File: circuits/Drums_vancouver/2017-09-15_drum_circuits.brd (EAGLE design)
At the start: 32 x 46 mm, 32 parts, among them IC2 MIC5225-5v, U2 ATMEGA328P_TQFP

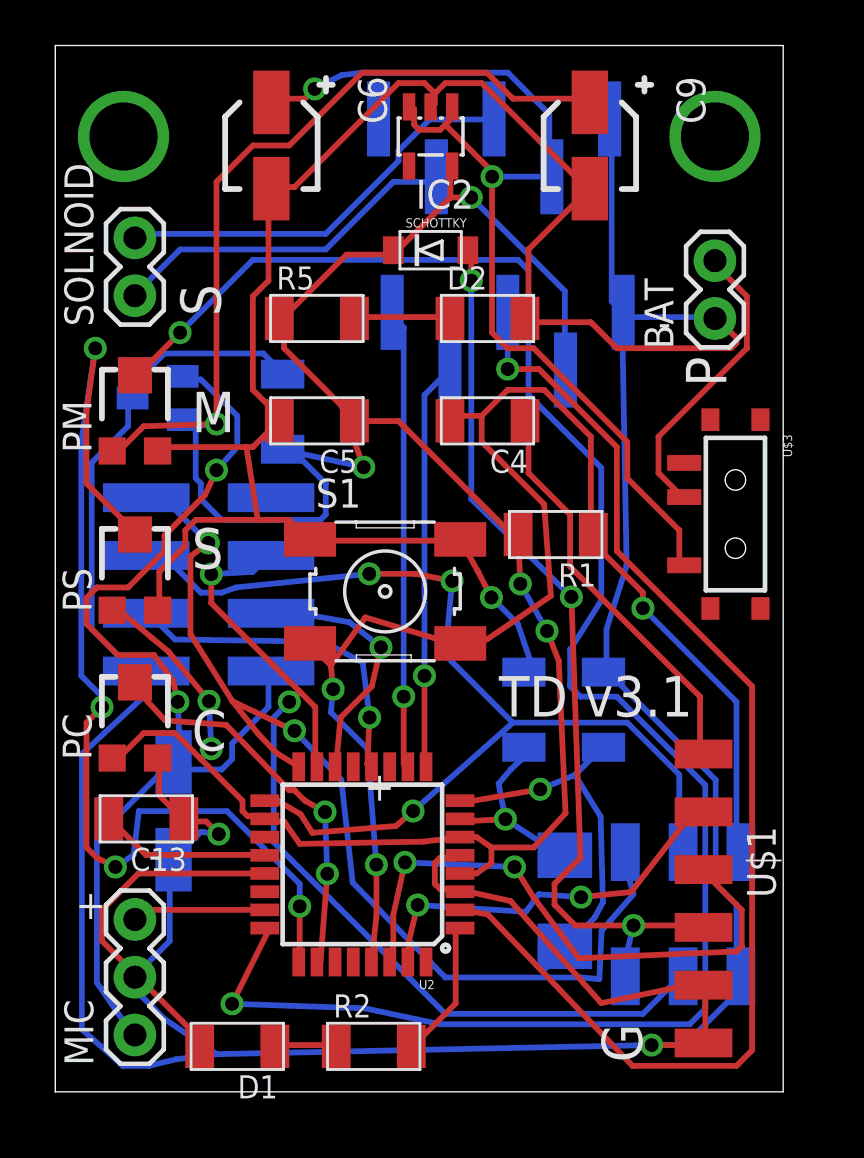
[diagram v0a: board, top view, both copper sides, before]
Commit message: updated slave, communication
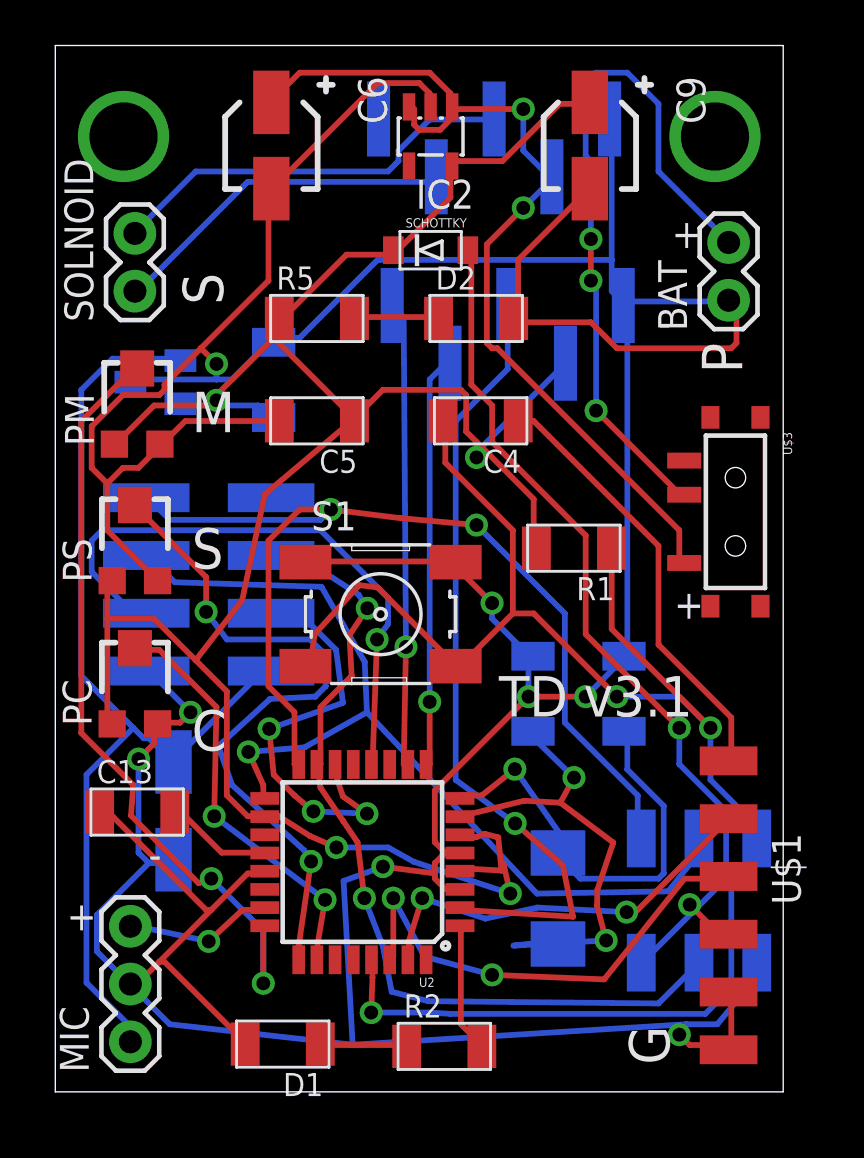
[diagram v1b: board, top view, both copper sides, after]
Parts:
- moved R2 3.10 mm to (17.1, 2.00)
- moved D1 2.00 mm to (10.0, 2.10)
- moved PC 1.50 mm to (3.50, 18.0)
- moved C3 1.46 mm to (9.60, 31.3)
- moved PS 1.30 mm to (3.50, 24.3)
- moved U$1 1.14 mm to (29.6, 8.20)
- moved C2 1.14 mm to (25.0, 17.5)
- moved S1 1.02 mm to (14.3, 21.0)
- moved R1 1.00 mm to (22.8, 23.9)
- moved BAT 1.00 mm to (29.6, 34.8)
- moved ISP 0.92 mm to (28.3, 8.60)
- moved C1 0.81 mm to (21.0, 17.5)
- moved VREG3.3 0.71 mm to (4.40, 31.2)
- moved C13 0.50 mm to (3.60, 12.3), turned to 0 degrees
- moved D2 0.50 mm to (18.5, 34.0)
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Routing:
- net PM: track 82.1 -> 34.6 mm
- net 5V: track 141.6 -> 110.6 mm, vias 7 -> 4
- net GND: track 252.8 -> 231.9 mm, vias 3 -> 8
- net ENABLE: track 53.7 -> 35.2 mm
- net BAT_IN: track 13.1 -> 31.3 mm, vias 0 -> 3
- net POT_S: track 48.1 -> 30.3 mm, vias 4 -> 2
- net XTAL1: track 9.36 -> 22.2 mm, vias 1 -> 2
- net CE: track 14.9 -> 26.5 mm
- net RST: track 64.6 -> 75.7 mm
- net CSN: track 11.1 -> 18.8 mm, vias 1 -> 3
- net SCK: track 46.7 -> 41.5 mm, vias 3 -> 1
- net VCC: track 46.6 -> 41.5 mm
- net MOSI: track 42.2 -> 37.9 mm
- net TX: track 25.6 -> 21.3 mm
- net N$9: track 7.58 -> 4.66 mm
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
